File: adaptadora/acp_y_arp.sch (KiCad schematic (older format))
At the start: 60 parts, among them J13 Conn_Coaxial, J14 Conn_Coaxial, J15 Conn_Coaxial, J16 Conn_Coaxial, J17 Conn_Coaxial, J18 Conn_Coaxial, J19 Conn_Coaxial, J20 Conn_Coaxial, J21 Conn_Coaxial, U10 SN74LVC2T45DCUR, U3 LM361MX_NOPB, U4 LM361MX_NOPB, U5 LM361MX_NOPB, U6 TLV2772IDR, U7 TLV2772IDR, U8 TLV2772IDR, U9 SN74LVC2T45DCUR

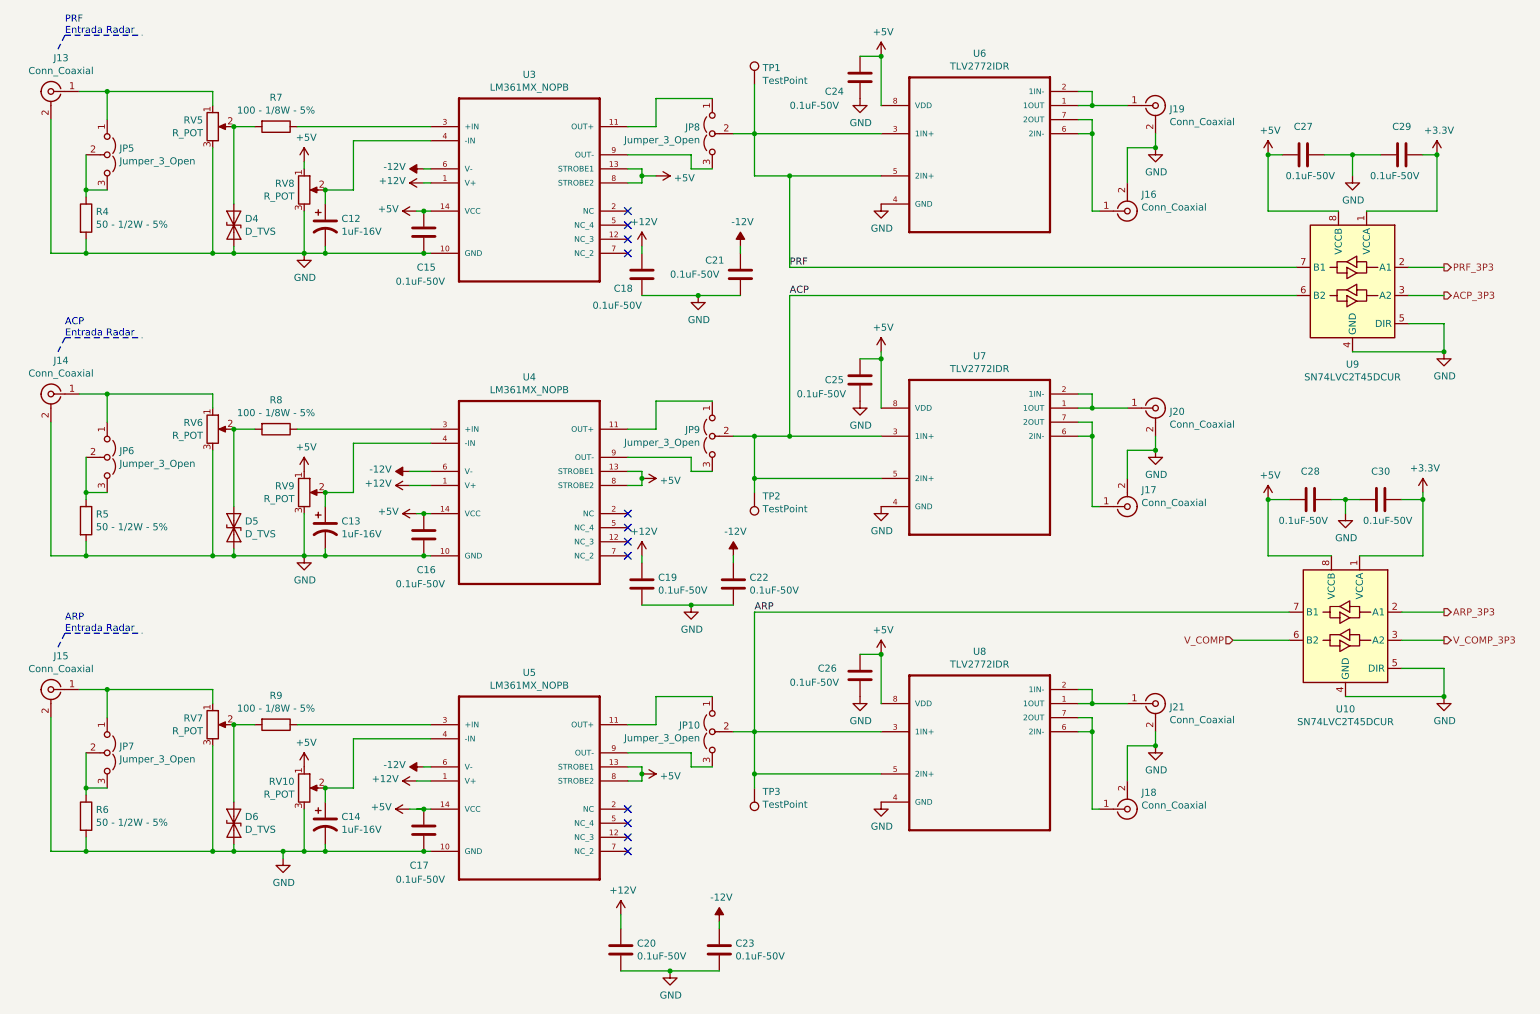
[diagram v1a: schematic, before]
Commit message: correcciones implementadas
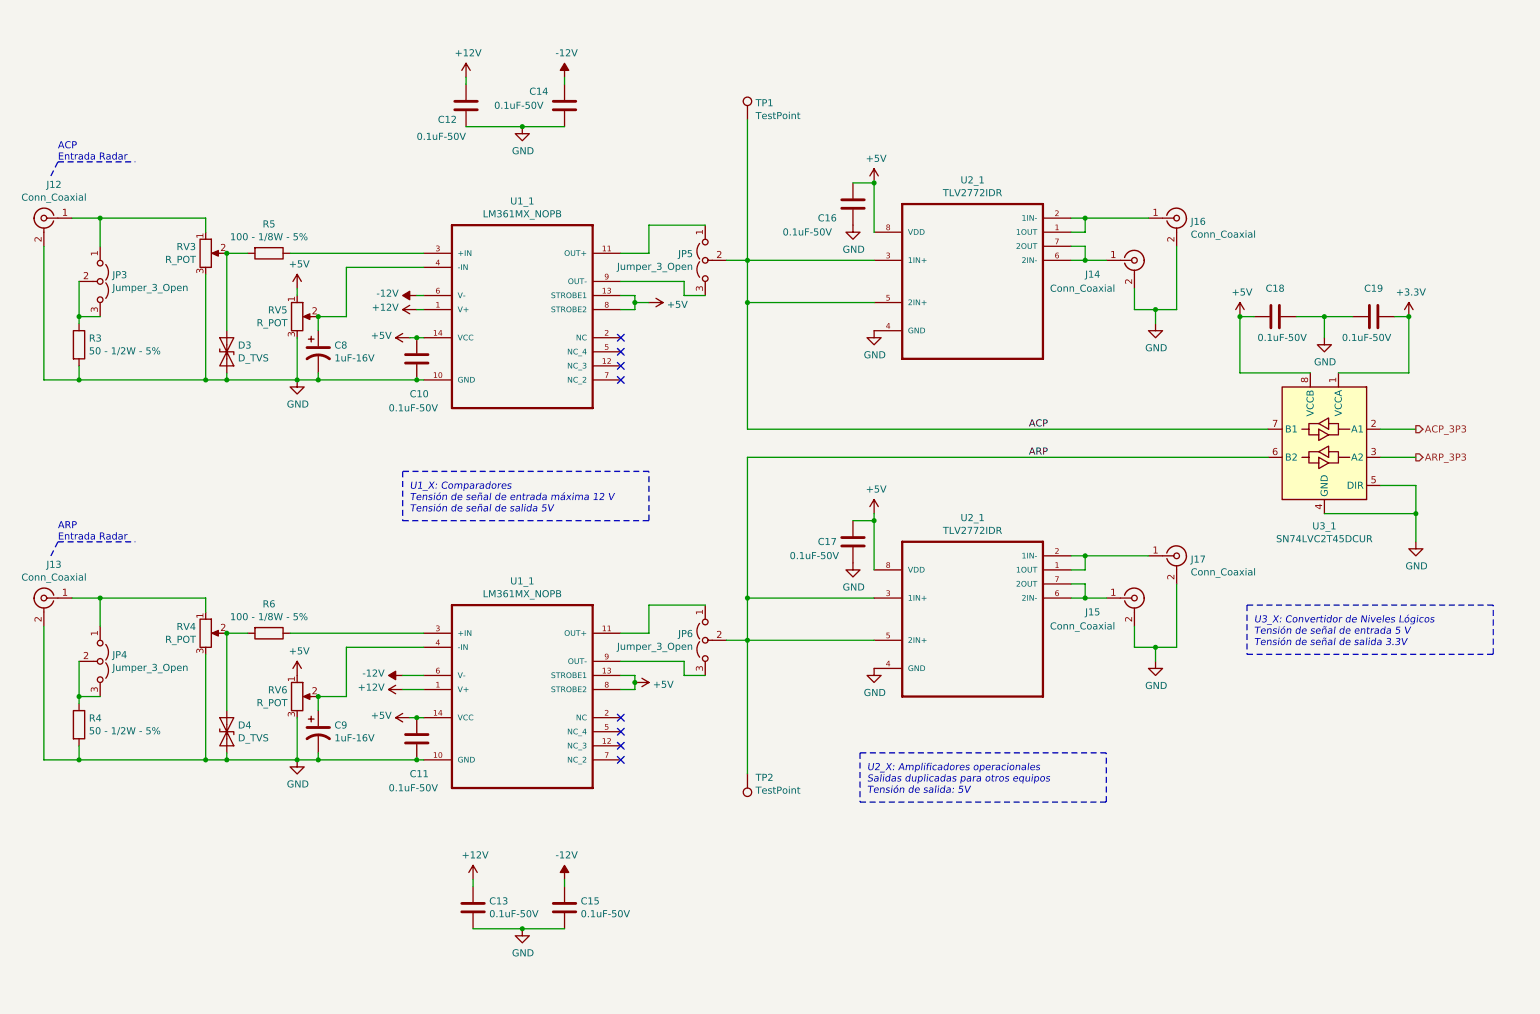
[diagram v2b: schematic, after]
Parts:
- removed C12, C13, C14: 1uF-16V, symbol Device:CP1
- removed C20, C21, C22, C23, C24, C25, C26, C27, C28, C29, C30: 0.1uF-50V, symbol Device:C
- removed D5, D6: D_TVS, symbol Device:D_TVS
- removed J18, J19, J20, J21: Conn_Coaxial, symbol Connector:Conn_Coaxial
- removed JP10, JP7, JP8, JP9: Jumper_3_Open, symbol Jumper:Jumper_3_Open
- removed R7, R8, R9: 100 - 1/8W - 5%, symbol Device:R
- removed RV10, RV7, RV8, RV9: R_POT, symbol Device:R_POT
- removed TP3: TestPoint, symbol Connector:TestPoint
- removed U10, U9: SN74LVC2T45DCUR, Package_SO:VSSOP-8_2.4x2.1mm_P0.5mm, symbol Logic_LevelTranslator:SN74LVC2T45DCUR
- removed U3, U4, U5: LM361MX_NOPB, SOIC127P600X175-14N, symbol sincronismo-rescue:LM361MX_NOPB-LM361MX_NOPB
- removed U6, U7, U8: TLV2772IDR, SOIC127P600X175-8N, symbol TLV2772IDR:TLV2772IDR
- added C10, C11, C12, C13, C14: 0.1uF-50V, symbol Device:C
- added C8, C9: 1uF-16V, symbol Device:CP1
- added D3: D_TVS, symbol Device:D_TVS
- added J12: Conn_Coaxial, symbol Connector:Conn_Coaxial
- added JP3, JP4: Jumper_3_Open, symbol Jumper:Jumper_3_Open
- added R3: 50 - 1/2W - 5%, symbol Device:R
- added RV3, RV4: R_POT, symbol Device:R_POT
- added U1_1 (x2): LM361MX_NOPB, SOIC127P600X175-14N, symbol sincronismo-rescue:LM361MX_NOPB-LM361MX_NOPB
- added U2_1 (x2): TLV2772IDR, SOIC127P600X175-8N, symbol TLV2772IDR:TLV2772IDR
- added U3_1: SN74LVC2T45DCUR, Package_SO:VSSOP-8_2.4x2.1mm_P0.5mm, symbol Logic_LevelTranslator:SN74LVC2T45DCUR
- R5, R6: value 50 - 1/2W - 5% -> 100 - 1/8W - 5%
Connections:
- net PRF is gone; now on net ACP: TP1.1
- net +12V: now also C12.1, C13.1, U1_1.1 (V+), U1_1.1 (V+); no longer C18.1, C19.1
- net +3V3: now also C19.1, U3_1.1 (VCCA)
- net +5V: now also C16.1, C17.1, C18.2, RV5.1, RV6.1, C10.2, C11.2, U1_1.13 (STROBE1), U1_1.13 (STROBE1), U1_1.14 (VCC), U1_1.14 (VCC), U1_1.8 (STROBE2), U1_1.8 (STROBE2), U2_1.8 (VDD), U2_1.8 (VDD), U3_1.8 (VCCB); no longer C15.2, C16.2, C17.2
- net -12V: now also C15.1, C14.1, U1_1.6 (V-), U1_1.6 (V-)
- net ACP: now also JP5.2 (C), U2_1.3 (1IN+), U2_1.5 (2IN+), U3_1.7 (B1); no longer TP2.1
- net ACP_3P3: now also U3_1.2 (A1)
- net ARP: now also JP6.2 (C), TP2.1, U2_1.3 (1IN+), U2_1.5 (2IN+), U3_1.6 (B2)
- net ARP_3P3: now also U3_1.3 (A2)
- net GND: now also C15.2, C16.2, C17.2, C18.1, C10.1, C11.1, C12.2, C13.2, C14.2, C8.2, C9.2, D3.2 (A2), J12.2 (Ext), R3.2, RV3.3, RV4.3, U1_1.10 (GND), U1_1.10 (GND), U2_1.4 (GND), U2_1.4 (GND), U3_1.4 (GND), U3_1.5 (DIR); no longer C15.1, C16.1, C17.1, C18.2, R5.2, R6.2
- net at RV5.2: now also C8.1, U1_1.4 (-IN); no longer D4.1 (A1)
- net at J16.1 (In): now also U2_1.1 (1OUT), U2_1.2 (1IN-)
- net at RV6.2: now also C9.1, U1_1.4 (-IN)
- net at J17.1 (In): now also U2_1.1 (1OUT), U2_1.2 (1IN-)
- net at J15.1 (In): now also U2_1.6 (2IN-), U2_1.7 (2OUT)
- net at R6.1: now also U1_1.3 (+IN)
- new net: J12.1 (In), JP3.1 (A), RV3.1
- new net: D3.1 (A1), R5.2, RV3.2
- new net: R5.1, U1_1.3 (+IN)
- new net: JP5.1 (A), U1_1.11 (OUT+)
- new net: JP5.3 (B), U1_1.9 (OUT-)
- new net: J14.1 (In), U2_1.6 (2IN-), U2_1.7 (2OUT)
- new net: JP6.1 (A), U1_1.11 (OUT+)
- new net: JP6.3 (B), U1_1.9 (OUT-)
- new net: JP3.2 (C), JP3.3 (B), R3.1
- new net: J13.1 (In), JP4.1 (A), RV4.1
- new net: JP4.2 (C), JP4.3 (B), R4.1
- new net: D4.1 (A1), R6.2, RV4.2
- no-connect marks 12 -> 8
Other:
- note added: "U1_X: Comparadores\nTensión de señal de entrada máxima 12 V\nTensión de señal de salida 5V"
- note added: "U2_X: Amplificadores operacionales\nSalidas duplicadas para otros equipos\nTensión de salida: 5V"
- note added: "U3_X: Convertidor de Niveles Lógicos\nTensión de señal de entrada 5 V\nTensión de señal de salida 3.3V"
- note removed: "PRF\nEntrada Radar"
